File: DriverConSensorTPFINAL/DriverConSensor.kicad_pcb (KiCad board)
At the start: 2 copper layers, 77 x 67 mm, 51 parts, among them J1 PULS1, J2 PULS2, J3 MotorT2, J4 MotorT1, J5 VIn+12, J6 Contac12V, J7 GND, K1 Switch de Encendido, K2 FRS10CS10-12V, K3 FRS10CS10-12V, Q1 BC337, Q2 BC337, SW1 SW_DIP_x06, U1 PIC12F675-IP, U2 L78L05, U3 ACS714T-30A

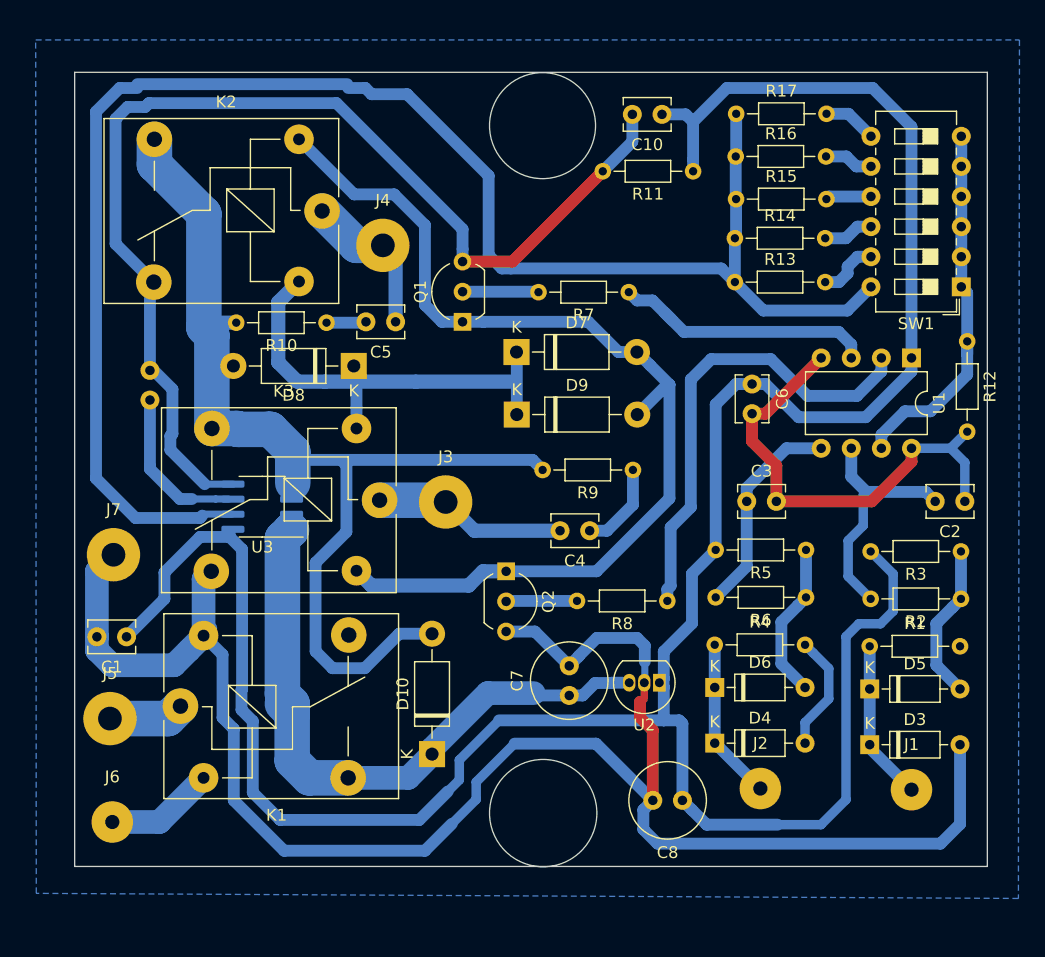
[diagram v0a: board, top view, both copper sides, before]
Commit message: actual4
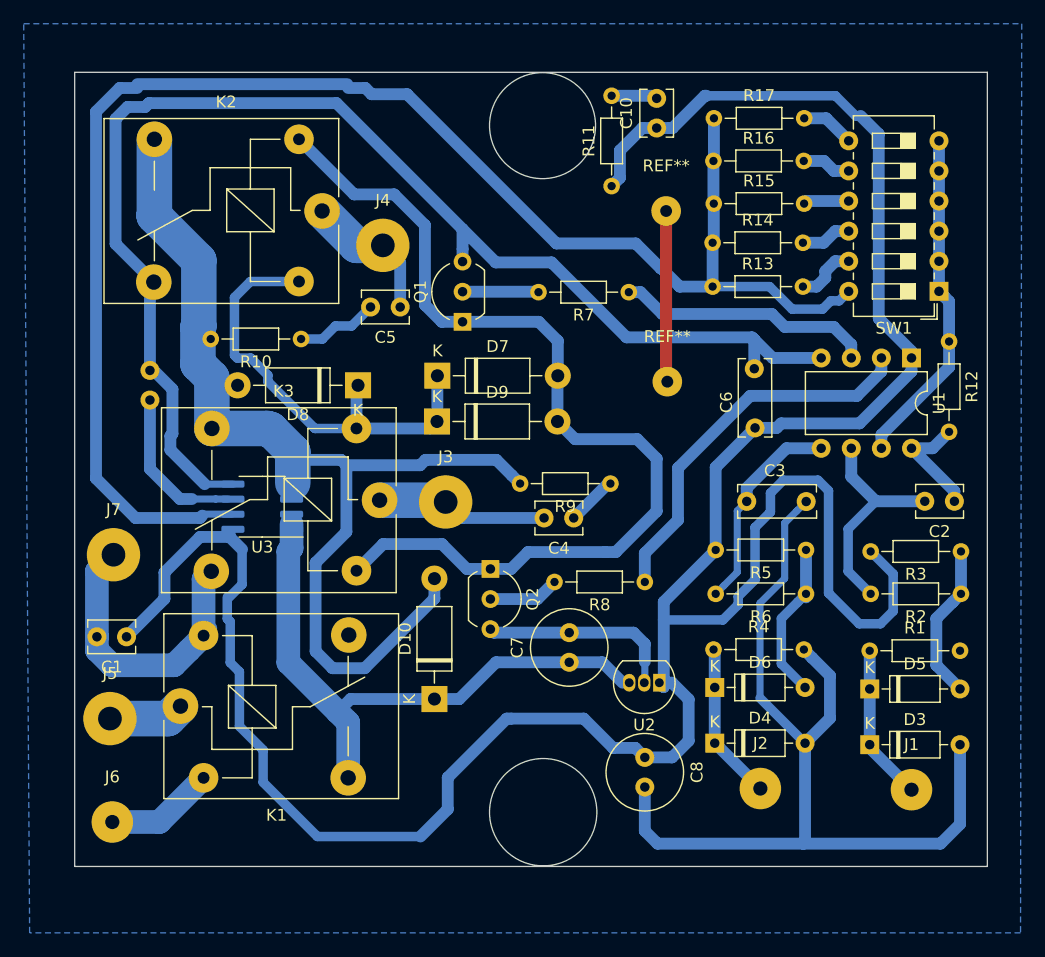
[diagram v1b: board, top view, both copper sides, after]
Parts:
- added REF**: SolderWirePad_1x01_Drill1mm, Connector_Wire:SolderWirePad_1x01_Drill1mm, F.Cu at (162.9, 74.7)
- added REF**: SolderWirePad_1x01_Drill1mm, Connector_Wire:SolderWirePad_1x01_Drill1mm, F.Cu at (163.0, 89.1)
- moved R11 6.99 mm to (158.3, 72.6), turned to 90 degrees
- moved D7 6.97 mm to (143.6, 88.6)
- moved D9 6.76 mm to (143.6, 92.5)
- moved C8 4.82 mm to (161.1, 120.8), turned to 270 degrees
- moved D10 4.65 mm to (143.3, 115.9)
- moved C6 3.71 mm to (170.4, 93.0), turned to 90 degrees
- moved C7 2.80 mm to (154.7, 112.8)
- moved R10 2.55 mm to (132.1, 85.5)
- moved R8 2.48 mm to (161.1, 106.0)
- moved R9 2.22 mm to (158.2, 97.7)
- moved R16 1.92 mm to (166.9, 70.5)
- moved SW1 1.92 mm to (185.9, 81.5)
- moved R15 1.92 mm to (166.9, 74.1)
- moved R13 1.92 mm to (166.8, 81.1)
- moved R14 1.92 mm to (166.8, 77.4)
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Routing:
- net GND: track 294.8 -> 262.1 mm
- net /GP5(PIN3PIC): track 39.6 -> 32.4 mm
- net Net-(R13-Pad1): track 136.9 -> 130.8 mm
- net Net-(D7-Pad2): track 87.1 -> 82.9 mm
- net /Relay2y3_NA: track 93.7 -> 89.5 mm
- net Net-(C5-Pad2): track 3.36 -> 6.98 mm
- net +12V: track 53.6 -> 50.1 mm
- net Net-(C4-Pad1): track 7.49 -> 4.30 mm
- net /GPIO0(PIN7PIC): track 31.9 -> 29.4 mm
- net Net-(C4-Pad2): track 16.4 -> 14.5 mm
- net Net-(C2-Pad2): track 20.8 -> 19.0 mm
- net +5V: track 221.6 -> 222.7 mm
- net /GP4(PIN2PIC): track 22.5 -> 21.7 mm
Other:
- outline, holes or cut-outs redrawn
